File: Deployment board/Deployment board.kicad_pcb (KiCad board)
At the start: 2 copper layers, 39.5 x 51 mm, 29 parts, among them J1 Conn_01x04, J2 Conn_01x04, J3 Conn_01x02, J4 Conn_01x02, J5 Conn_01x02, J6 REMOVE BEFORE FLIGHT, M1 Motor_Servo, Q1 IRLR7843, Q2 IRLR7843, Q3 To be determined

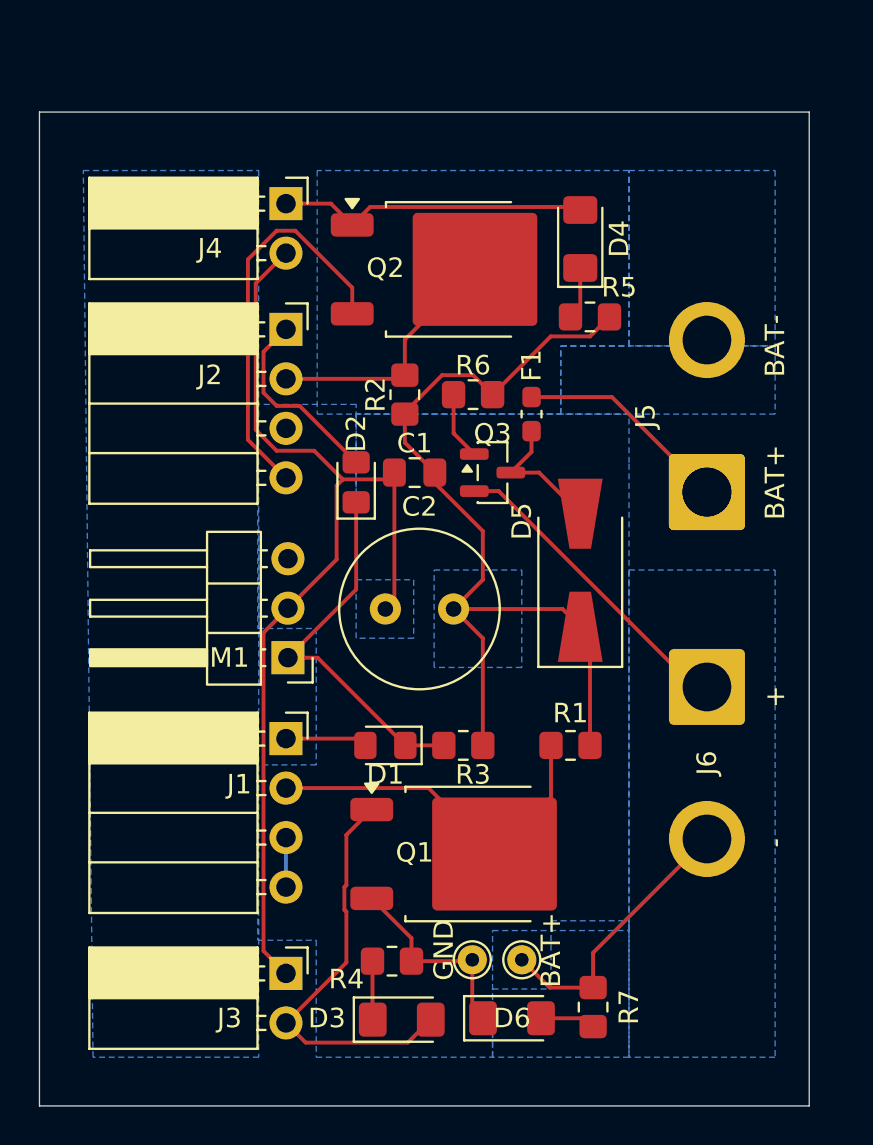
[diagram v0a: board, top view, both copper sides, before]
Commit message: jpush
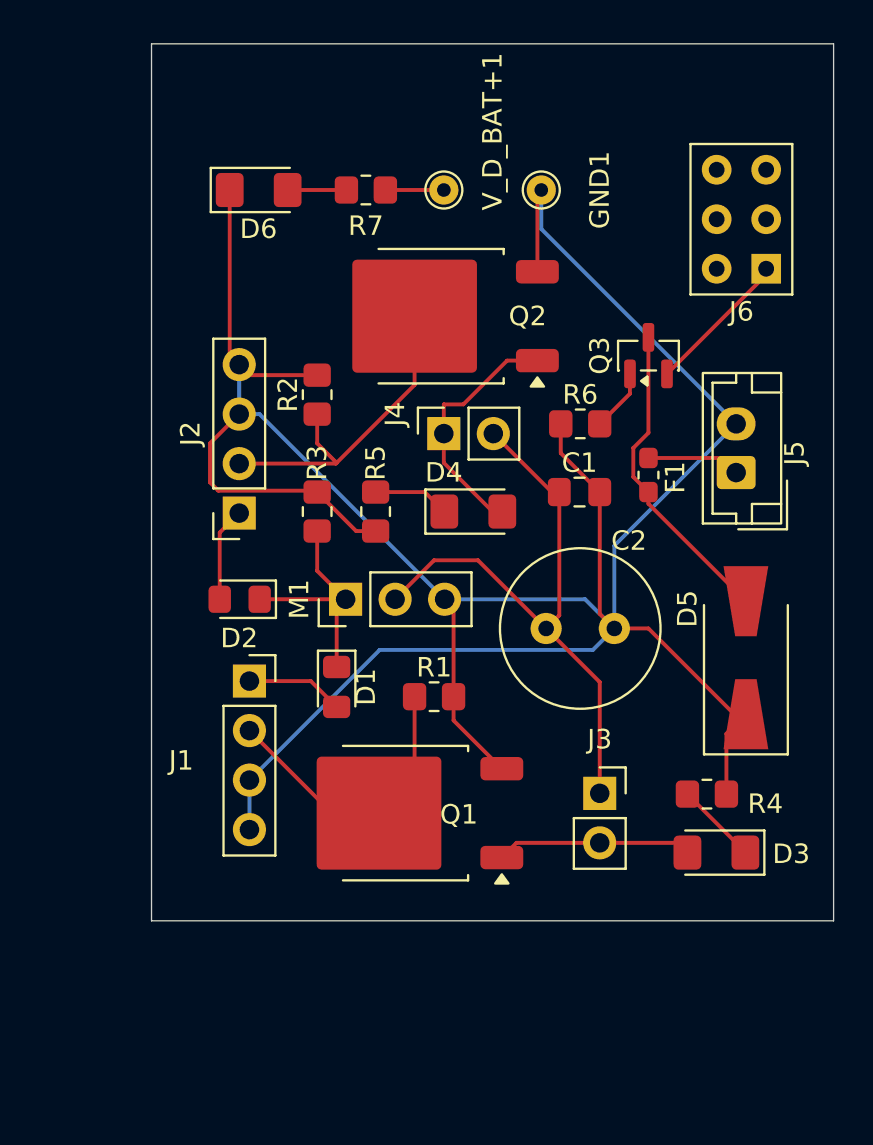
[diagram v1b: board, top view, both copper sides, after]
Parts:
- removed ?: , 
- removed BAT+, GND: TestPoint, TestPoint:TestPoint_THTPad_D1.5mm_Drill0.7mm
- added GND1: TestPoint, TestPoint:TestPoint_THTPad_D1.5mm_Drill0.7mm, F.Cu at (40.5, 107.5)
- added V_D_BAT+1: TestPoint, TestPoint:TestPoint_THTPad_D1.5mm_Drill0.7mm, F.Cu at (35.5, 107.5)
- J1, J2: footprint Connector_PinSocket_2.54mm:PinSocket_1x04_P2.54mm_Horizontal -> Connector_PinSocket_2.54mm:PinSocket_1x04_P2.54mm_Vertical
- J3, J4: footprint Connector_PinSocket_2.54mm:PinSocket_1x02_P2.54mm_Horizontal -> Connector_PinSocket_2.54mm:PinSocket_1x02_P2.54mm_Vertical
- J5: footprint Connector_Wire:SolderWire-2sqmm_1x02_P7.8mm_D2mm_OD3.9mm -> Connector_JST:JST_EH_B2B-EH-A_1x02_P2.50mm_Vertical
- J6: footprint Connector_Wire:SolderWire-2sqmm_1x02_P7.8mm_D2mm_OD3.9mm -> Button_Switch_THT:SW_NKK_G1xJP
- M1: footprint Connector_PinHeader_2.54mm:PinHeader_1x03_P2.54mm_Horizontal -> Connector_PinHeader_2.54mm:PinHeader_1x03_P2.54mm_Vertical
- moved D6 44.4 mm to (26.0, 107.5)
- moved R7 43.5 mm to (31.5, 107.5), turned to 0 degrees
- moved J6 21.7 mm to (52.0, 111.5), turned to 180 degrees
- moved J3 18.6 mm to (43.5, 138.5)
- moved R4 18.3 mm to (49.0, 138.5)
- moved D3 18.3 mm to (49.5, 141.5), turned to 180 degrees
- moved D4 15.0 mm to (37.0, 124.0), turned to 0 degrees
- moved R5 14.9 mm to (32.0, 124.0), turned to -90 degrees
- moved J4 14.3 mm to (35.5, 120.0), turned to 90 degrees
- moved R3 14.2 mm to (29.0, 124.0), turned to 90 degrees
- moved Q3 10.0 mm to (46.0, 116.0), turned to 90 degrees
- moved J2 9.73 mm to (25.0, 124.1), turned to 180 degrees
- moved D5 9.61 mm to (51.0, 131.5)
- moved C1 8.52 mm to (42.5, 123.0)
- moved D2 8.47 mm to (25.0, 128.5), turned to 180 degrees
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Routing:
- net GND: track 80.6 -> 145.4 mm
- net V_Ｄ_BAT+: track 52.7 -> 31.5 mm
- net Net-(D3-A): track 21.2 -> 9.34 mm
- net V_D_BAT+: track 14.3 -> 3.00 mm
- net Net-(D5-A2): track 7.00 -> 16.3 mm
- net Main_AV_FIRE: track 18.9 -> 10.1 mm
- net Net-(J6-A): track 16.1 -> 7.51 mm
- net Net-(D1-K): track 19.3 -> 12.2 mm
- net Net-(J5-Pin_1): track 11.0 -> 4.81 mm
- net Backup_AV_PWM_Servo: track 9.96 -> 4.83 mm
- net Backup_AV_FIRE: track 13.1 -> 17.1 mm
- net Net-(D4-A): track 16.0 -> 12.8 mm
- net Net-(D4-K): track 2.72 -> 3.94 mm
- net Net-(D3-K): track 3.01 -> 4.21 mm
- net Main_AV_PWM_Servo: track 4.22 -> 5.02 mm
- removed copper zone on B.Cu, net GND
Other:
- board size 39.5 x 51 mm -> 35 x 45 mm
- board text removed: "+"
- board text removed: "-"
- board text removed: "BAT+"
- board text removed: "BAT-"
